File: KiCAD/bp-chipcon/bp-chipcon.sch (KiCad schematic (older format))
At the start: 15 parts, among them J1 Conn_Coaxial, M1 BLUE_PILL, U1 74HC86

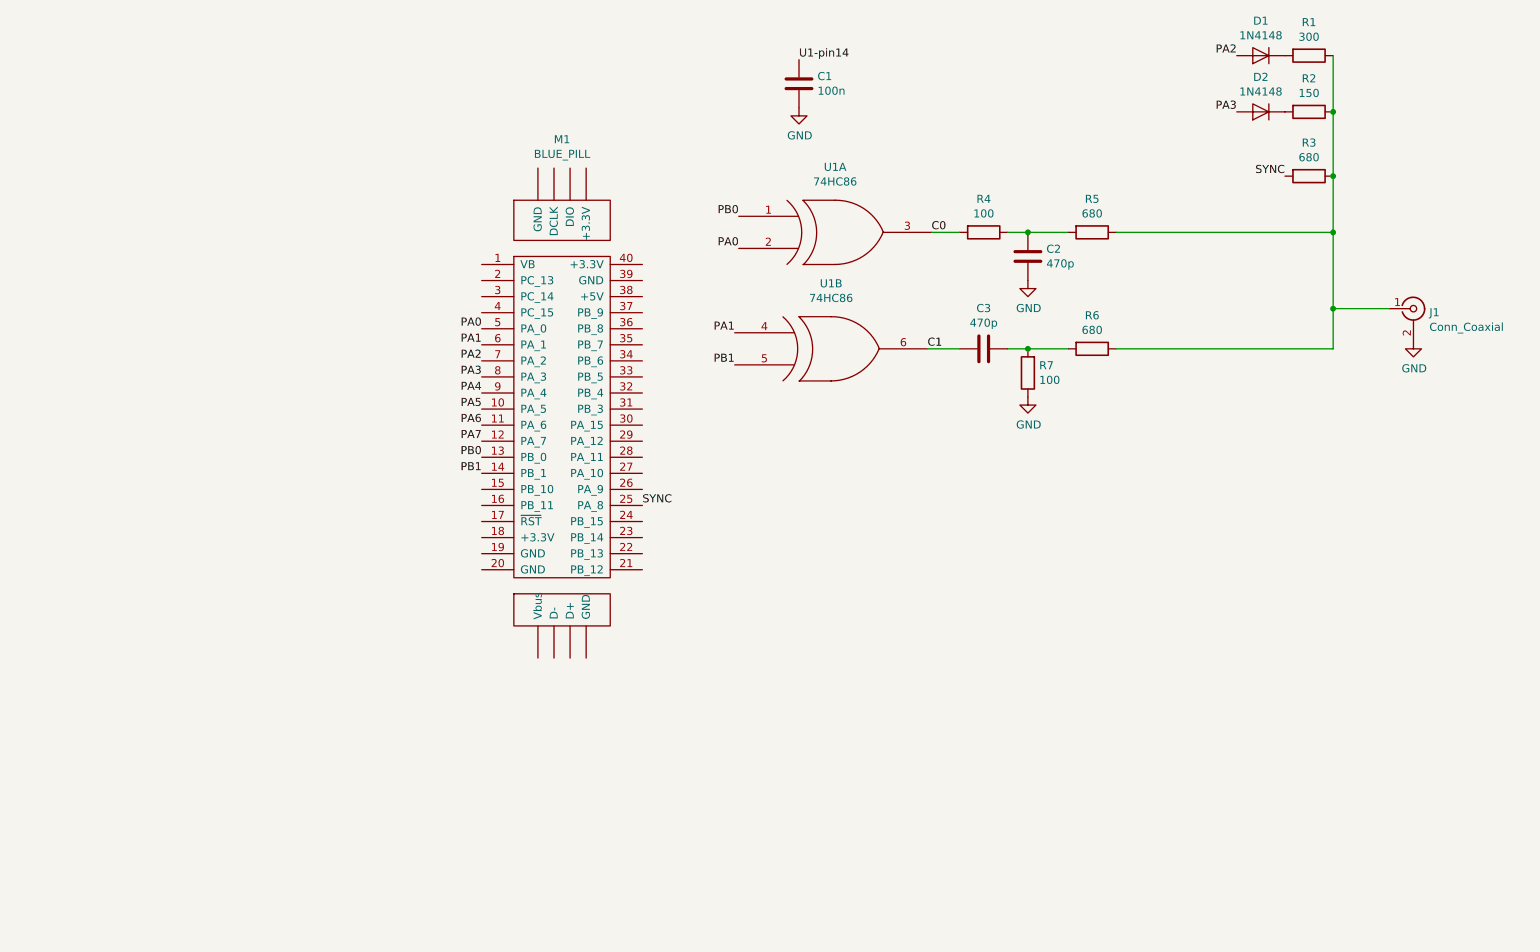
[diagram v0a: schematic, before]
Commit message: modification to schematic
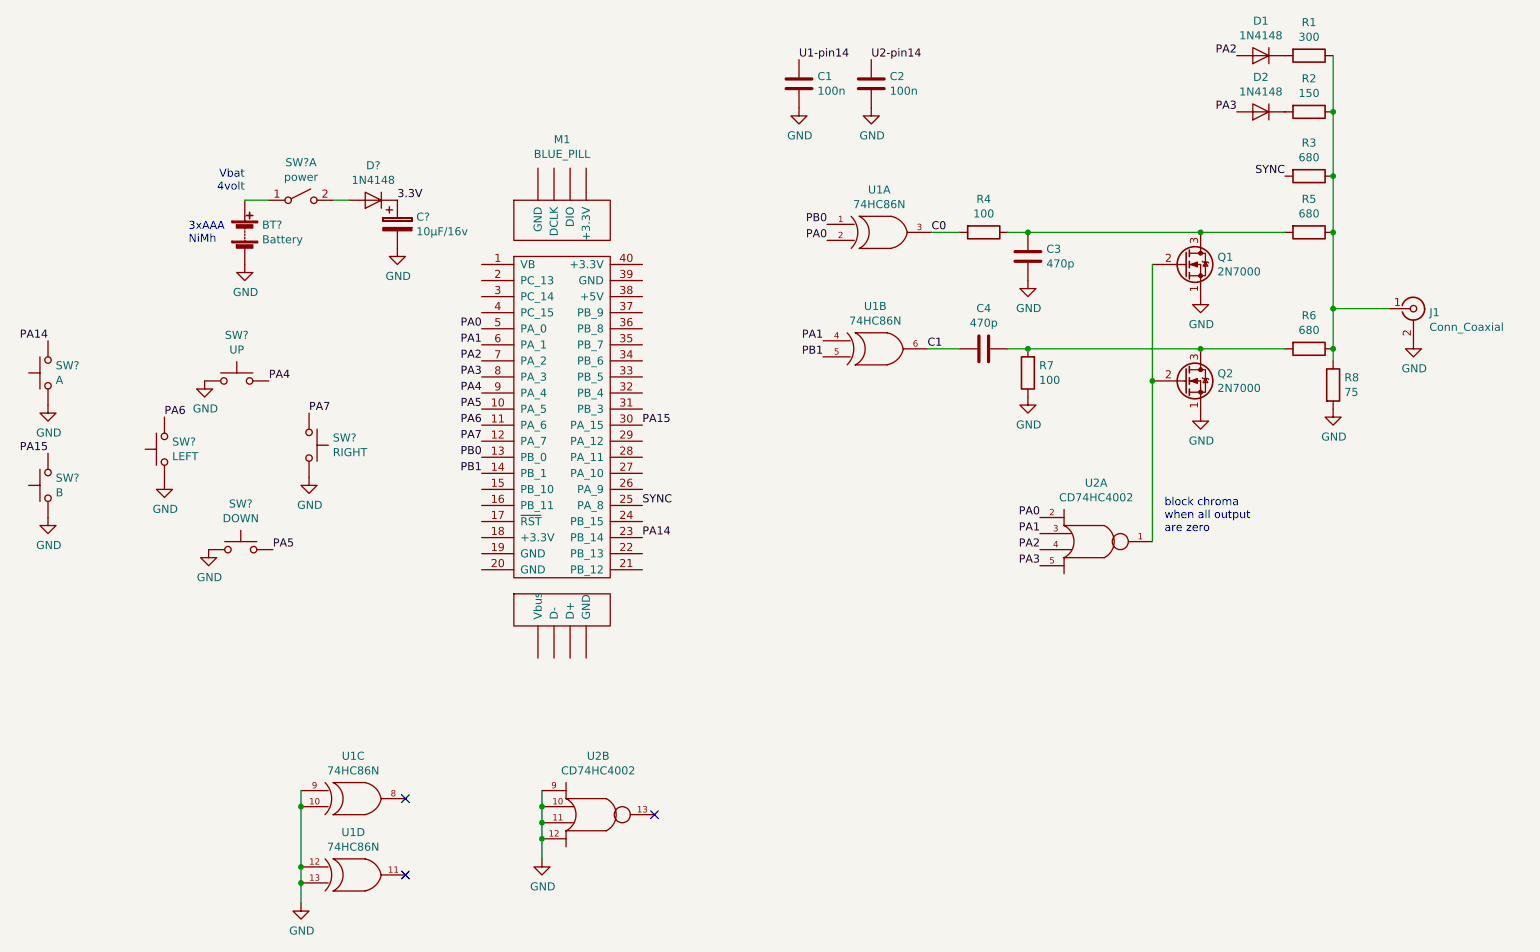
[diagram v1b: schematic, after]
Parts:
- removed U1: 74HC86, symbol 74xx:74HC86
- added BT?: Battery, symbol device:Battery
- added C2: 100n, symbol device:C
- added C?: 10µF/16v, symbol device:CP
- added D?: 1N4148, symbol device:D
- added Q1, Q2: 2N7000, TO_SOT_Packages_THT:TO-92_Molded_Narrow, symbol transistors:2N7000
- added R8: 75, symbol device:R
- added SW?: power, symbol switches:SW_DPST_x2
- added SW?: LEFT, symbol switches:SW_Push
- added SW?: RIGHT, symbol switches:SW_Push
- added SW?: UP, symbol switches:SW_Push
- added SW?: DOWN, symbol switches:SW_Push
- added SW?: A, symbol switches:SW_Push
- added SW?: B, symbol switches:SW_Push
- added U1: 74HC86N, symbol Personal_KiCAD:74HC86N
- added U2: CD74HC4002, symbol Personal_KiCAD:CD74HC4002
- renumbered C2 to C3, C3 to C4
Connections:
- net C0: now also U1.3
- net C1: now also U1.6
- net GND: now also BT?.2 (-), C2.2, C?.2, Q1.1 (S), Q2.1 (S), R8.2, SW?.1, SW?.1, SW?.1, SW?.1, SW?.1, SW?.2, U1.10, U1.12, U1.13, U1.9, U2.10, U2.11, U2.12, U2.9
- net PA0: now also U1.2, U2.2
- net PA1: now also U1.4, U2.3
- net PA2: now also U2.4
- net PA3: now also U2.5
- net PA4: now also SW?.2
- net PA5: now also SW?.2
- net PA6: now also SW?.2
- net PA7: now also SW?.1
- net PB0: now also U1.1
- net PB1: now also U1.5
- net PA14: now reaches M1.23 (PB_14)
- net PA14: now also SW?.2
- net PA15: now reaches M1.30 (PA_15)
- net PA15: now also SW?.2
- net at C3.1, R4.1, R5.2: now also Q1.3 (D)
- net at C4.1, R6.2, R7.2: now also Q2.3 (D)
- net at J1.1 (In), R1.1, R2.1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: now also R8.1
- new net: Q1.2 (G), Q2.2 (G), U2.1
- new net: BT?.1 (+), SW?.1 (A)
- new net: D?.2 (A), SW?.2 (B)
- new net 3.3V: C?.1, D?.1 (K)
- new net U2-pin14: C2.1
- no-connect marks 0 -> 3
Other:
- note added: "3xAAA\nNiMh"
- note added: "Vbat\n4volt\n"
- note added: "block chroma\nwhen all output\nare zero"
- moved on the sheet: R5, R6
